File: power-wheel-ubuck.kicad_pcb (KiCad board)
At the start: 2 copper layers, 23 parts, among them J1 CONN_01X02_MALE, J10 TEST_1P, J2 TEST_1P, J3 TEST_1P, J4 CONN_01X03_MALE, J5 TEST_1P, J6 TEST_1P, J7 TEST_1P, J8 TEST_1P, J9 CONN_01X02_MALE, U1 TPS563200DDCR

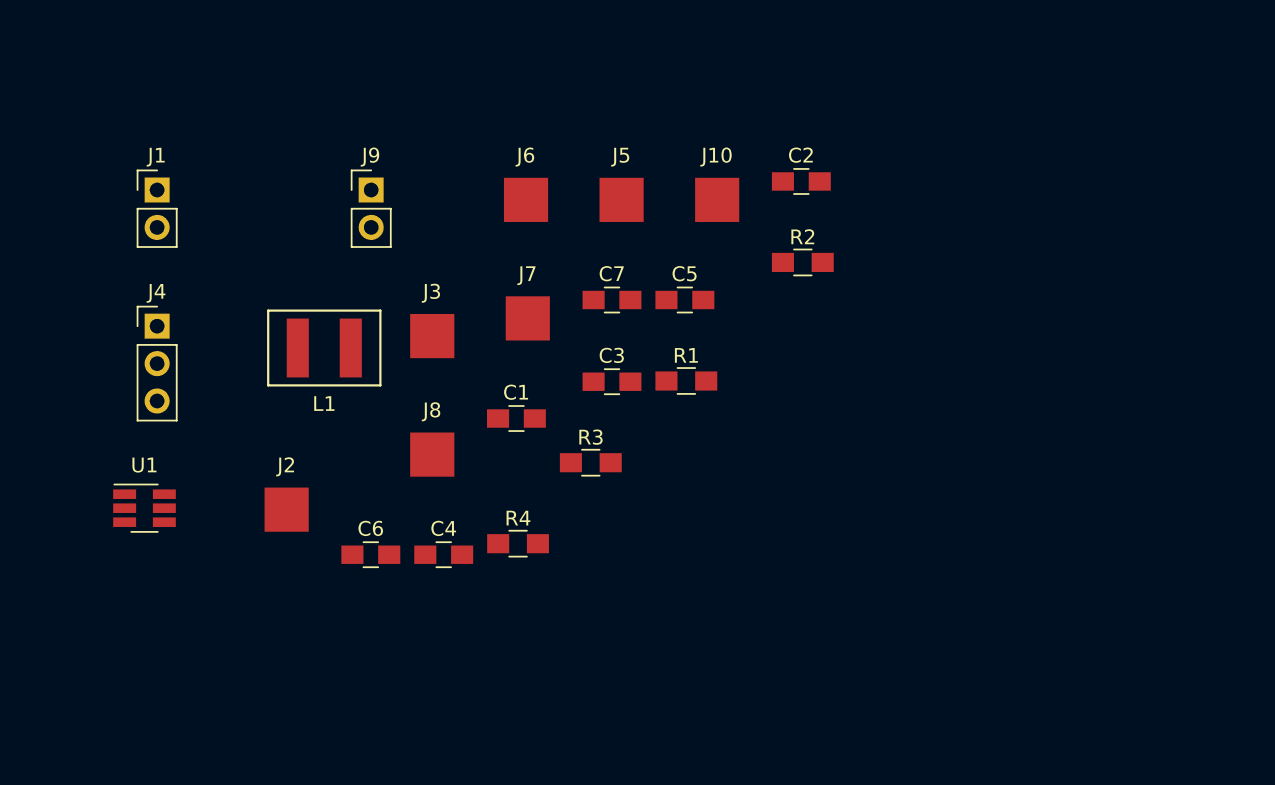
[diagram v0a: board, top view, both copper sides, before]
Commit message: Initial layout start
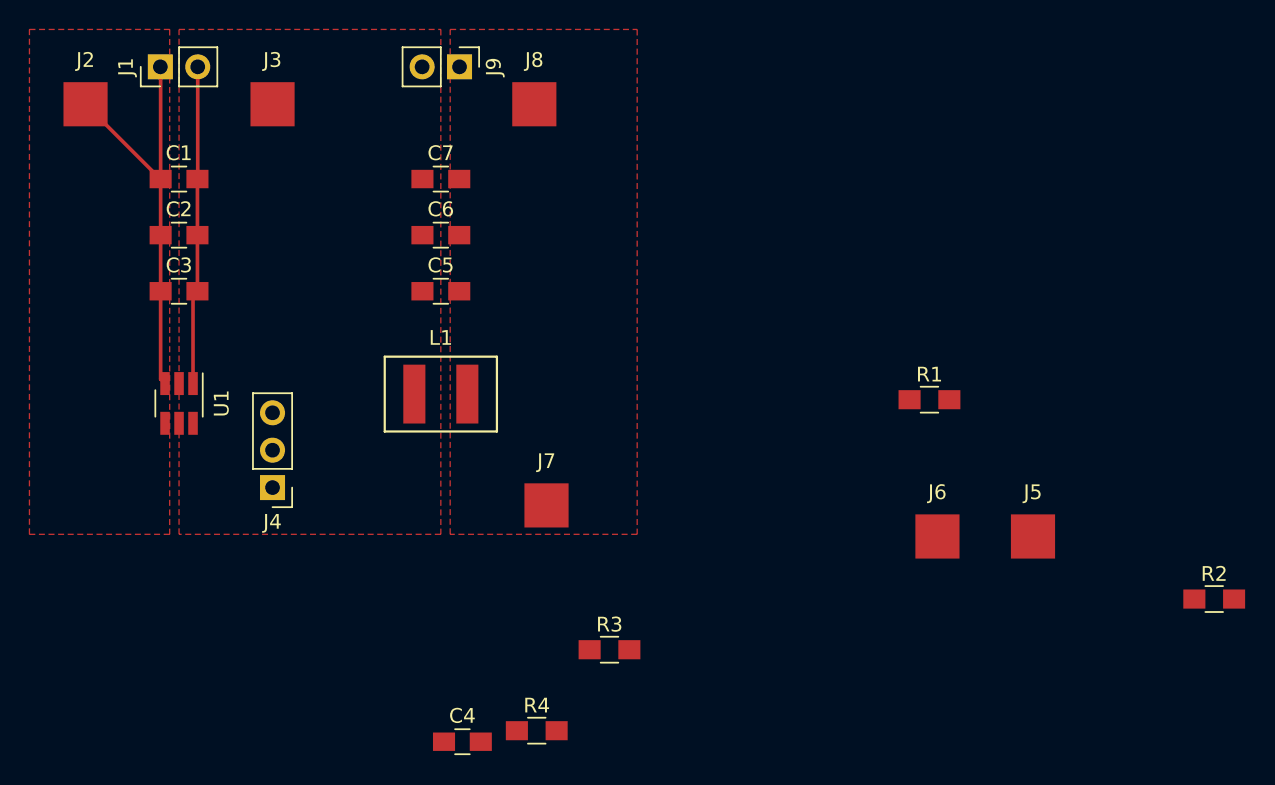
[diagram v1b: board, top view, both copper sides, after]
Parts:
- removed J10: TEST_1P, Measurement_Points:Measurement_Point_Square-SMD-Pad_Big
- moved C2 42.4 mm to (137.2, 90.2)
- moved J5 36.1 mm to (195.2, 110.6)
- moved J6 36.1 mm to (188.7, 110.6)
- moved R2 36.1 mm to (207.5, 114.9)
- moved J2 30.7 mm to (130.8, 81.3)
- moved C3 30.0 mm to (137.2, 94.0)
- moved C1 28.1 mm to (137.2, 86.4)
- moved J8 24.8 mm to (161.3, 81.3)
- moved C6 22.2 mm to (154.9, 90.2)
- moved J3 19.1 mm to (143.5, 81.3)
- moved C5 16.6 mm to (154.9, 94.0)
- moved R1 16.6 mm to (188.1, 101.3)
- moved C7 14.2 mm to (154.9, 86.4)
- moved J4 13.5 mm to (143.5, 107.3), turned to 180 degrees
- moved C4 12.8 mm to (156.4, 124.6)
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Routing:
- net Net-(C1-Pad1): track 0.00 -> 28.8 mm
- net GND: track 0.00 -> 21.6 mm
- added copper zone on F.Cu, net GND
- added copper zone on F.Cu, net Net-(C1-Pad1)
- added copper zone on F.Cu, net Net-(C5-Pad2)
